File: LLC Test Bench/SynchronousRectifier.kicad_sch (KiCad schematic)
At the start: 1 part, among them U2 UCC24624DR

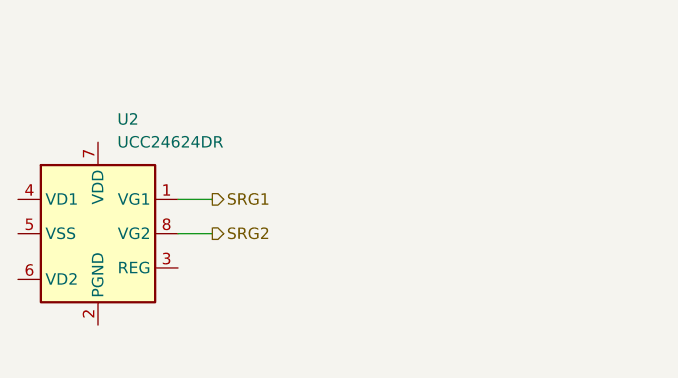
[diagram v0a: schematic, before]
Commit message: Rev 1.7
- Finished Sync Rect
- updated root page to match sync rect
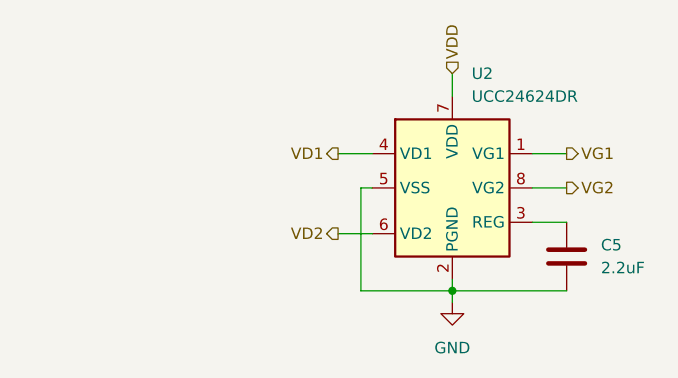
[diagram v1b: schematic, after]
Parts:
- added C5: 2.2uF, symbol Device:C
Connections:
- net GND: now reaches U2.2 (PGND)
- net GND: now also U2.5 (VSS), C5.2
- net at U2.3 (REG): now also C5.1
- net VD1: now reaches U2.4 (VD1)
- net VD2: now reaches U2.6 (VD2)
- net VDD: now reaches U2.7 (VDD)
- net SRG1 renamed VG1
- net SRG2 renamed VG2
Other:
- moved on the sheet: U2
